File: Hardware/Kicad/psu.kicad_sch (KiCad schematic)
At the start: 21 parts, among them J7 Barrel_Jack_Switch, U7 TPS62160DSG, U8 TPS7A2033PDBVR, U9 TPS7A2018PDBVR

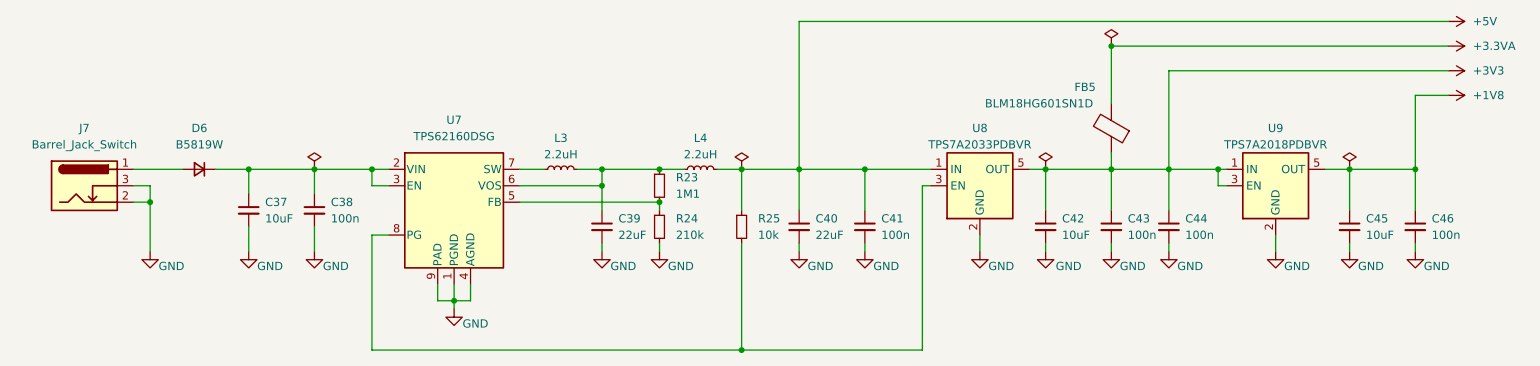
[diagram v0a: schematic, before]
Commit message: Small hardware update
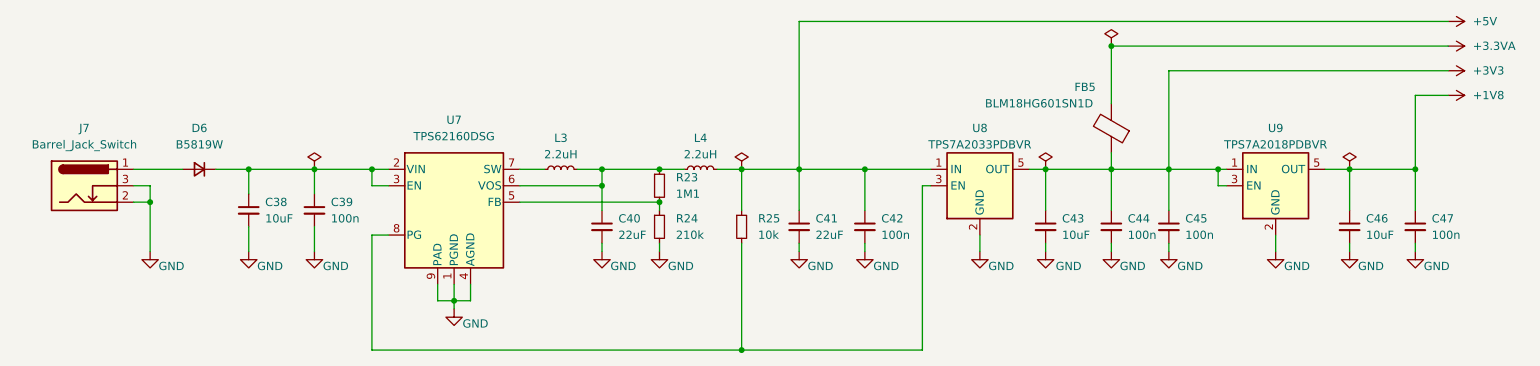
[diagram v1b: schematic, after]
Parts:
- renumbered C37 to C38, C38 to C39, C39 to C40, C40 to C41, C41 to C42, C42 to C43, C43 to C44, C44 to C45, C45 to C46, C46 to C47
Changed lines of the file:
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@@
 		(dnp no)
 		(fields_autoplaced yes)
-		(property "Reference" "C40"
+		(property "Reference" "C41"
 			(at 148.59 53.3462 0)
 			(show_name no)
@@
 			(project "PAL-sign"
 				(path "/5e4b4b86-505e-4573-b1db-0e4430e7f8ee"
-					(reference "C40")
+					(reference "C41")
 					(unit 1)
 				)
@@
 		(dnp no)
 		(fields_autoplaced yes)
-		(property "Reference" "C44"
+		(property "Reference" "C45"
 			(at 205.74 53.3462 0)
 			(show_name no)
@@
 			(project "PAL-sign"
 				(path "/5e4b4b86-505e-4573-b1db-0e4430e7f8ee"
-					(reference "C44")
+					(reference "C45")
 					(unit 1)
 				)
@@
 		(dnp no)
 		(fields_autoplaced yes)
-		(property "Reference" "C46"
+		(property "Reference" "C47"
 			(at 243.84 53.3462 0)
 			(show_name no)
@@
 			(project "PAL-sign"
 				(path "/5e4b4b86-505e-4573-b1db-0e4430e7f8ee"
-					(reference "C46")
+					(reference "C47")
 					(unit 1)
 				)
@@
 		(dnp no)
 		(fields_autoplaced yes)
-		(property "Reference" "C43"
+		(property "Reference" "C44"
 			(at 196.85 53.3462 0)
 			(show_name no)
@@
 			(project "PAL-sign"
 				(path "/5e4b4b86-505e-4573-b1db-0e4430e7f8ee"
-					(reference "C43")
+					(reference "C44")
 					(unit 1)
 				)
@@
 		(dnp no)
 		(fields_autoplaced yes)
-		(property "Reference" "C42"
+		(property "Reference" "C43"
 			(at 186.69 53.3462 0)
 			(show_name no)
@@
 			(project "PAL-sign"
 				(path "/5e4b4b86-505e-4573-b1db-0e4430e7f8ee"
-					(reference "C42")
+					(reference "C43")
 					(unit 1)
 				)
@@
 		(dnp no)
 		(fields_autoplaced yes)
-		(property "Reference" "C41"
+		(property "Reference" "C42"
 			(at 158.75 53.3462 0)
 			(show_name no)
@@
 			(project "PAL-sign"
 				(path "/5e4b4b86-505e-4573-b1db-0e4430e7f8ee"
-					(reference "C41")
+					(reference "C42")
 					(unit 1)
 				)
@@
 		(dnp no)
 		(fields_autoplaced yes)
-		(property "Reference" "C45"
+		(property "Reference" "C46"
 			(at 233.68 53.3462 0)
 			(show_name no)
@@
 			(project "PAL-sign"
 				(path "/5e4b4b86-505e-4573-b1db-0e4430e7f8ee"
-					(reference "C45")
+					(reference "C46")
 					(unit 1)
 				)
@@
 		(dnp no)
 		(fields_autoplaced yes)
-		(property "Reference" "C37"
+		(property "Reference" "C38"
 			(at 63.5 50.8062 0)
 			(show_name no)
@@
 			(project "PAL-sign"
 				(path "/5e4b4b86-505e-4573-b1db-0e4430e7f8ee"
-					(reference "C37")
+					(reference "C38")
 					(unit 1)
 				)
@@
 		(dnp no)
 		(fields_autoplaced yes)
-		(property "Reference" "C38"
+		(property "Reference" "C39"
 			(at 73.66 50.8062 0)
 			(show_name no)
@@
 			(project "PAL-sign"
 				(path "/5e4b4b86-505e-4573-b1db-0e4430e7f8ee"
-					(reference "C38")
+					(reference "C39")
 					(unit 1)
 				)
@@
 		(dnp no)
 		(fields_autoplaced yes)
-		(property "Reference" "C39"
+		(property "Reference" "C40"
 			(at 118.11 53.3462 0)
 			(show_name no)
@@
 			(project "PAL-sign"
 				(path "/5e4b4b86-505e-4573-b1db-0e4430e7f8ee"
-					(reference "C39")
+					(reference "C40")
 					(unit 1)
 				)
